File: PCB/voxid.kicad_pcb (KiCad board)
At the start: 2 copper layers, 51 parts, among them J1 Audio, J2 HPF_O, J3 LPFO, J4 Offset, J5 v3.3, J6 AudioOut, U1 TL072, U2 TL072, U3 TL072, U4 LM1117T-3.3

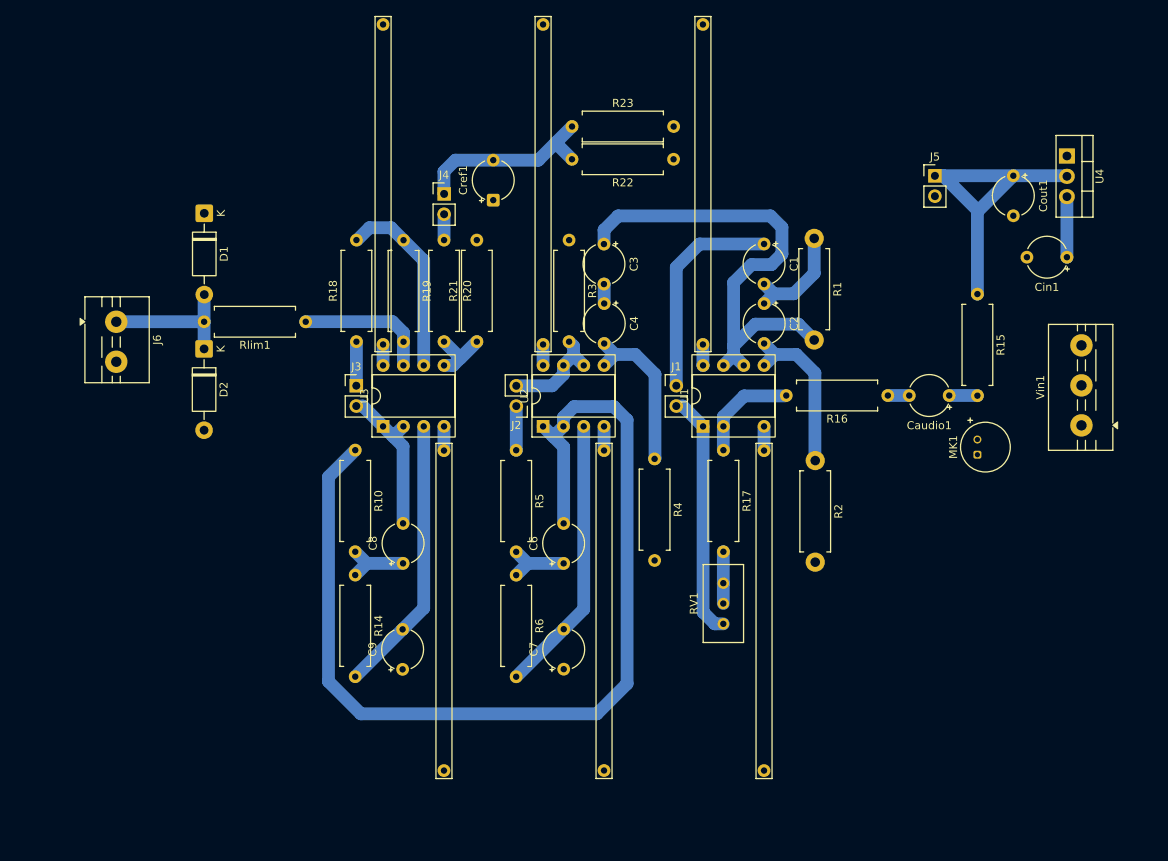
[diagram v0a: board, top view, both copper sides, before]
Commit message: pcb: Creacion de geber para cnc
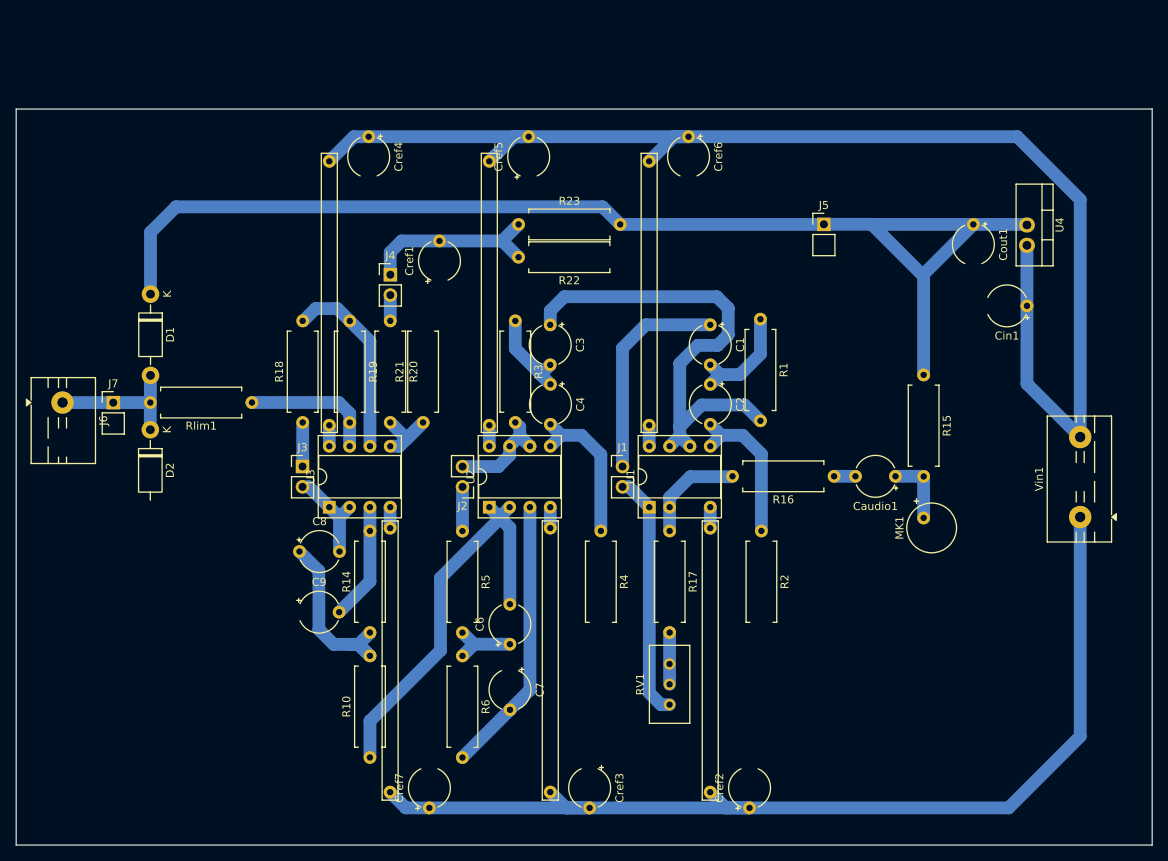
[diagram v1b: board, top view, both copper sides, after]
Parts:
- added Cref2: 100nF, Capacitor_THT:CP_Radial_Tantal_D5.0mm_P5.00mm, F.Cu at (91.7, 87.4)
- added Cref3: 100nF, Capacitor_THT:CP_Radial_Tantal_D5.0mm_P5.00mm, F.Cu at (71.7, 82.4)
- added Cref4: 100nF, Capacitor_THT:CP_Radial_Tantal_D5.0mm_P5.00mm, F.Cu at (44.1, 3.46)
- added Cref5: 100nF, Capacitor_THT:CP_Radial_Tantal_D5.0mm_P5.00mm, F.Cu at (64.1, 8.46)
- added Cref6: 100nF, Capacitor_THT:CP_Radial_Tantal_D5.0mm_P5.00mm, F.Cu at (84.0, 3.46)
- added Cref7: 100nF, Capacitor_THT:CP_Radial_Tantal_D5.0mm_P5.00mm, F.Cu at (51.7, 87.4)
- added J7: v3.3, Connector_PinHeader_2.54mm:PinHeader_1x02_P2.54mm_Vertical, F.Cu at (12.1, 36.7)
- moved R10 38.5 mm to (44.2, 81.1), turned to 90 degrees
- moved J5 15.1 mm to (101.0, 14.4)
- moved C9 14.8 mm to (35.4, 62.9), turned to 0 degrees
- moved R23 13.9 mm to (62.8, 14.4)
- moved R22 13.9 mm to (75.5, 18.5)
- moved C8 13.0 mm to (35.4, 55.3), turned to 0 degrees
- moved C6 12.1 mm to (61.7, 66.9)
- moved R18 12.1 mm to (35.8, 39.2)
- moved R5 12.1 mm to (55.8, 52.8)
- moved TP1 12.1 mm to (79.1, 39.5)
- moved TP2 12.1 mm to (39.1, 39.5)
- moved TP3 12.1 mm to (59.1, 39.5)
- moved D1 12.1 mm to (16.8, 23.1)
- moved C1 12.1 mm to (86.8, 27.0)
- moved C3 12.1 mm to (66.8, 27.0)
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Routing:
- net +12V: track 15.5 -> 175.1 mm
- net -12V: track 9.06 -> 137.6 mm
- net +3.3V: track 39.5 -> 150.1 mm
- net Net-(U2A--): track 129.2 -> 51.7 mm
- net Net-(U3A-+): track 34.8 -> 14.7 mm
- net Net-(C8-Pad1): track 8.64 -> 23.9 mm
- net Net-(C3-Pad2): track 2.45 -> 11.5 mm
- net Net-(J3-Pin_2): track 19.4 -> 12.3 mm
- net Net-(MK1-+): track 3.53 -> 8.71 mm
- net Net-(U2B-+): track 20.5 -> 19.4 mm
- net Vref: track 24.0 -> 23.2 mm
- net Net-(U1B-+): track 20.2 -> 19.5 mm
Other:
- board outline added: 142 x 92 mm
